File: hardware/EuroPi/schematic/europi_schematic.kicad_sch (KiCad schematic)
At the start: 88 parts, among them J1 Conn_02x05_Odd_Even, J10 Output 6 Jack, J11 Conn_01x04_Pin, J2 Conn_01x04_Pin, J3 Output 1 Jack, J4 Output 4 Jack, J5 Analogue Input Jack, J6 Output 2 Jack, J7 Output 5 Jack, J8 Digital Input Jack, J9 Output 3 Jack, Q1 2N2222, SW1 SW_Push, SW2 SW_Push, U2 PICO_RP2040, U3 TL074, U4 TL074, U5 MCP6002-xSN, U6 L7805

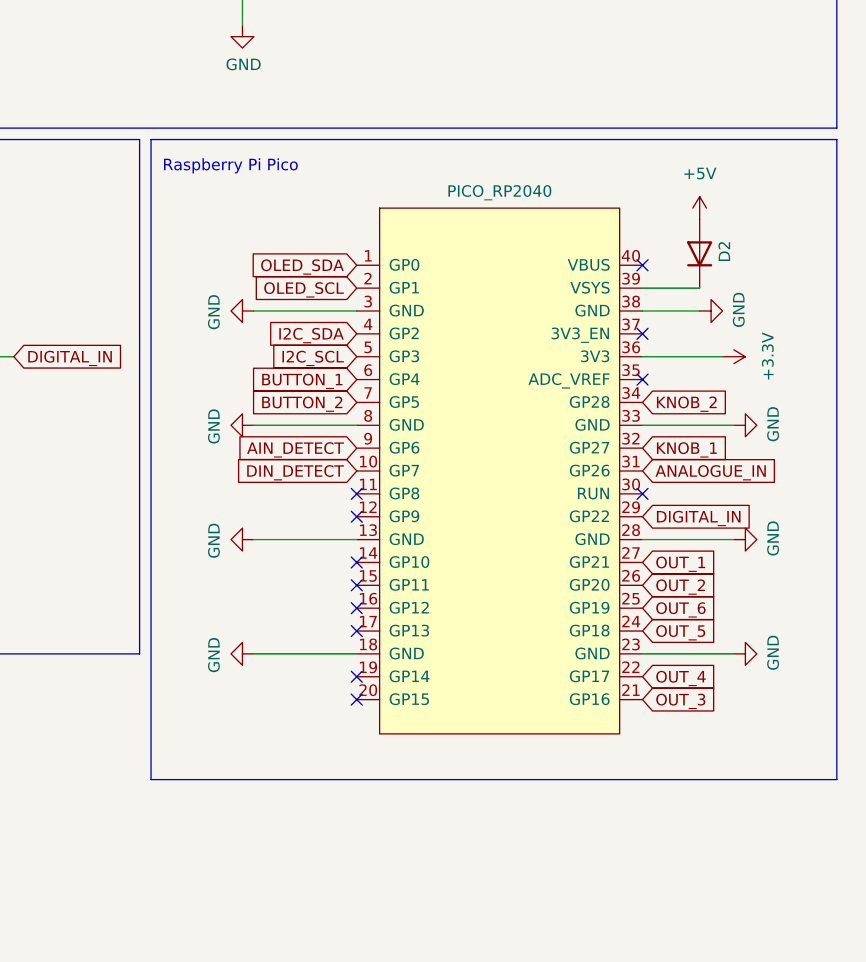
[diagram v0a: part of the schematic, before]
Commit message: ordered rev 1
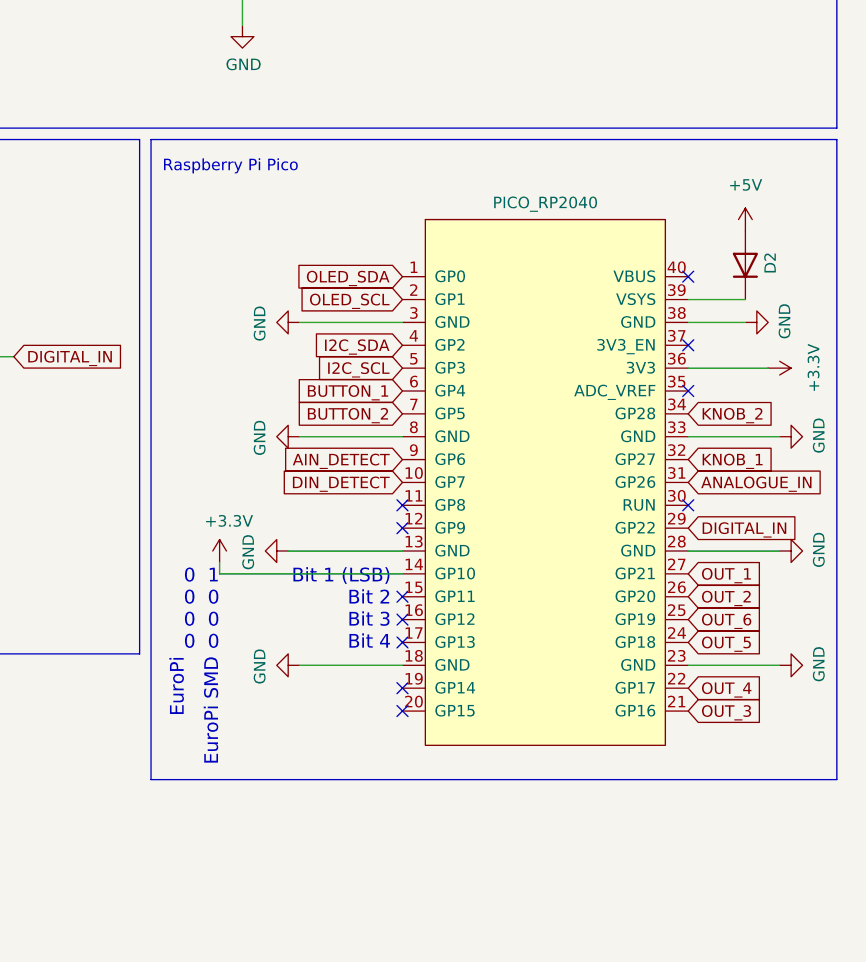
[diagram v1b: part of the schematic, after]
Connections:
- net +3.3V: now also U2.14 (GP10)
- no-connect marks 24 -> 23
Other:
- note added: "0 1 0 0 0 0 0 0"
- note added: "Bit 1 (LSB) Bit 2 Bit 3 Bit 4"
- note added: "EuroPi"
- note added: "EuroPi SMD"
- moved on the sheet: D2
